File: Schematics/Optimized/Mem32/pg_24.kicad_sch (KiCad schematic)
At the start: 8 parts, among them U2508 F04, U2509 F86, U2510 F86, U2526 F521, U2527 F299, U30 XHASH, U47 XPAR32, U54 XADRPAR

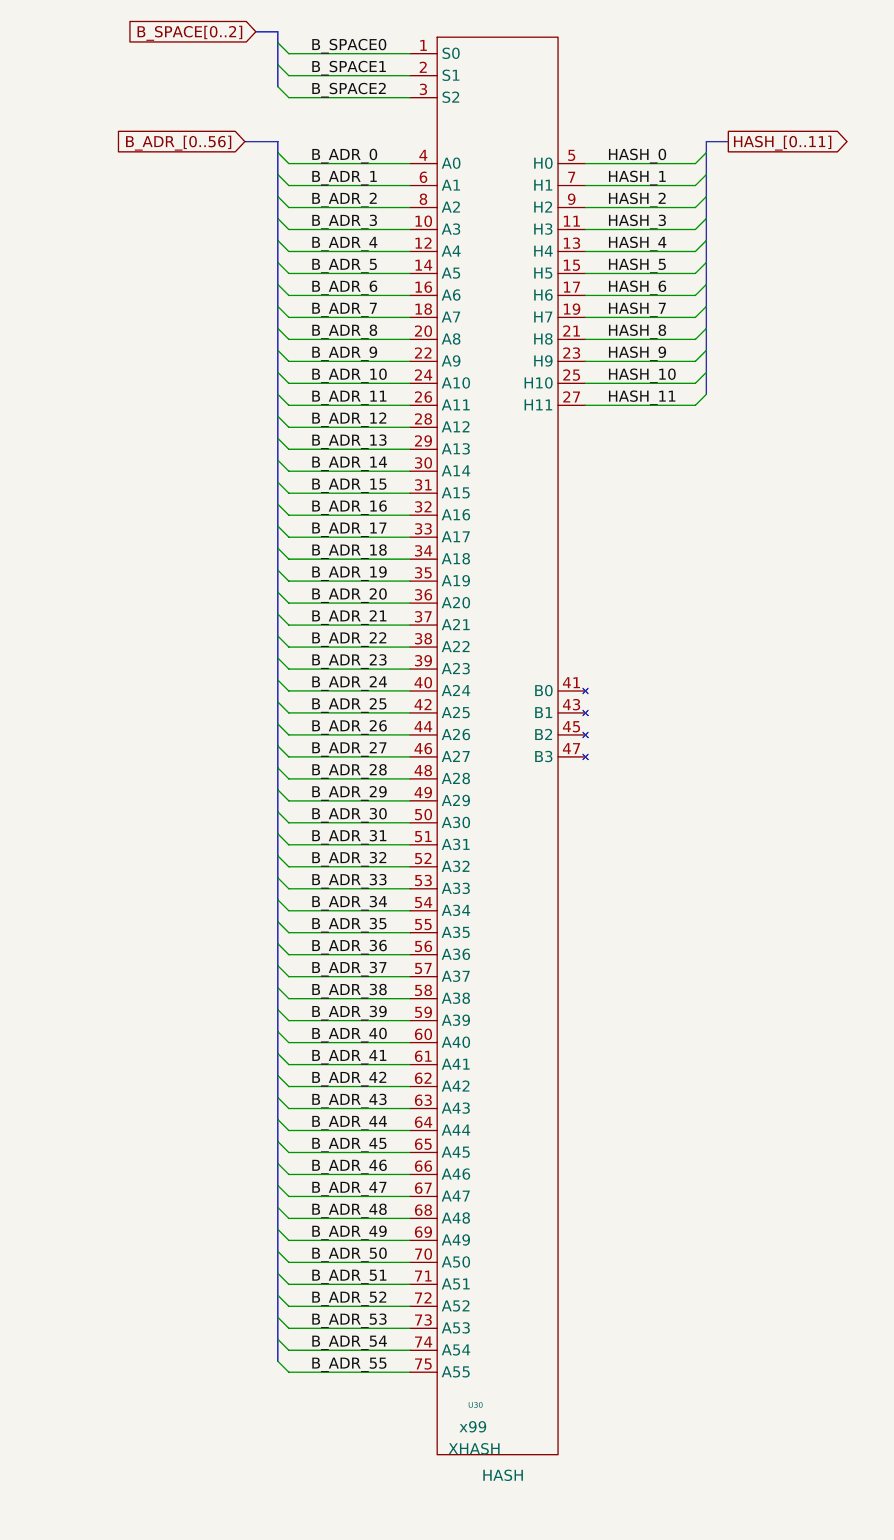
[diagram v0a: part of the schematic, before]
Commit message: MEM32 improvements
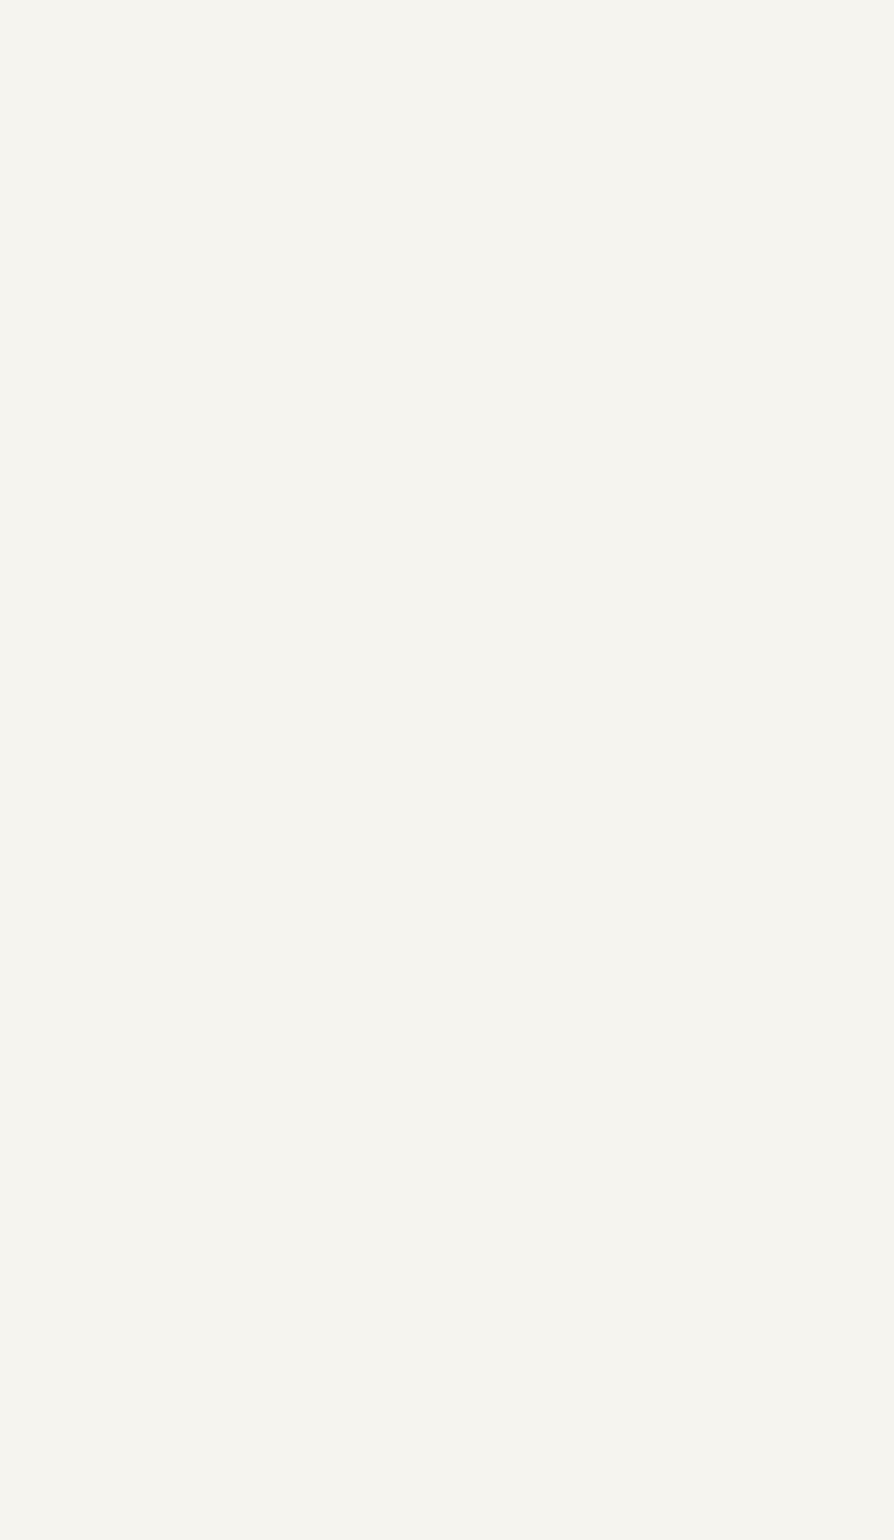
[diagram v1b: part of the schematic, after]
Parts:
- removed U30: XHASH, symbol r1000:XHASH
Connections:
- no-connect marks 19 -> 15
